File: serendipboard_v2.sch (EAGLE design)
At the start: 18 parts, among them IC1 TP4056, IC2 DW01A, Q1 FS8205A, Q2 DMP3056LSD, Q3 DMP3056LSD

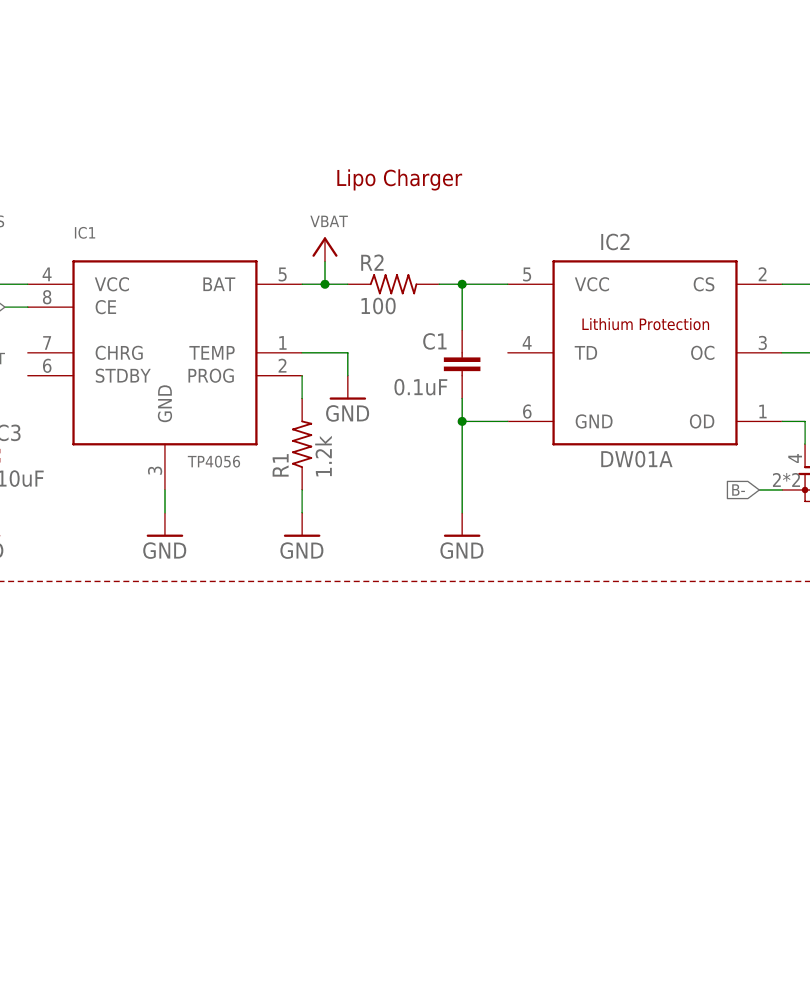
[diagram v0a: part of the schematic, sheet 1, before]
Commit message: Update serendipboard_v2.sch
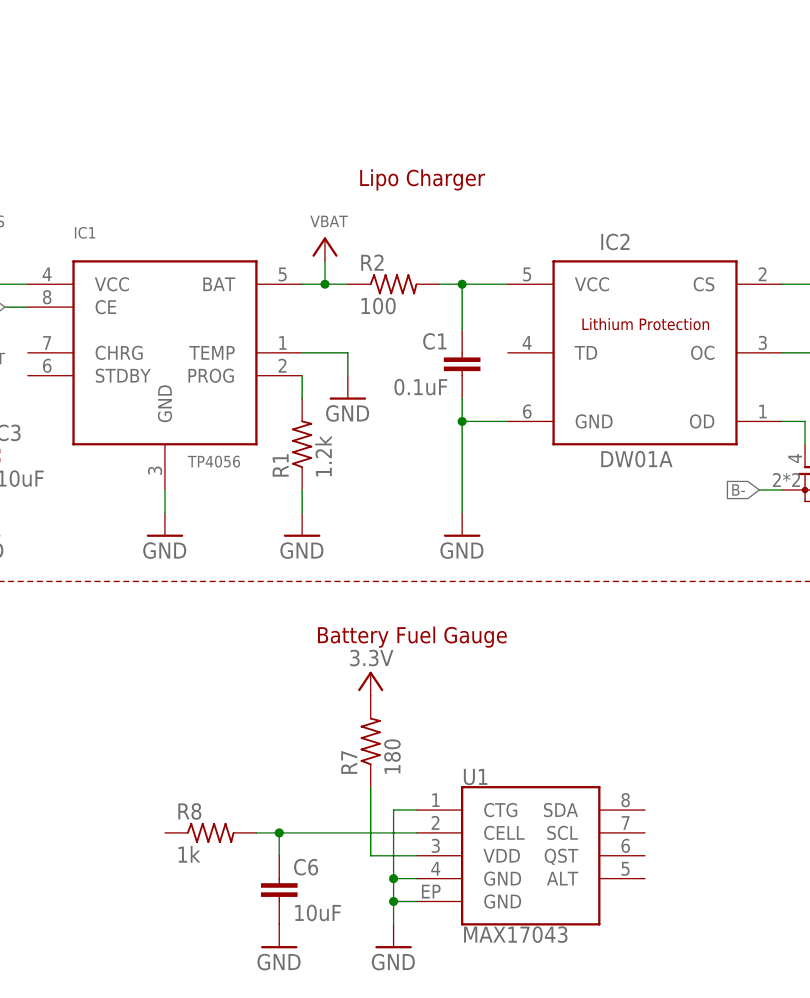
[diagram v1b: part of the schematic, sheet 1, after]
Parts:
- added C6: 10uF, rcl:C-EUC0805
- added R7: 180, rcl:R-US_R0805
- added R8: 1k, rcl:R-US_R0805
- added U1: MAX17043, SparkFun-IC-Power:MAX1704X
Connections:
- new net N$6: R7.1, U1.VDD
- new net N$7: C6.1, R8.2, U1.CELL
- net GND: now also C6.2, U1.CTG, U1.GND@4, U1.GND@EP
- net VCC: now also R7.2
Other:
- note added: "Battery Fuel Gauge"
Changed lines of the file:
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@@
 <layer number="112" name="tSilk" color="7" fill="1" visible="no" active="yes"/>
 <layer number="113" name="ReferenceLS" color="7" fill="1" visible="no" active="no"/>
+<layer number="114" name="Badge_Outline" color="7" fill="1" visible="yes" active="yes"/>
+<layer number="115" name="ReferenceISLANDS" color="7" fill="1" visible="yes" active="yes"/>
 <layer number="116" name="Patch_BOT" color="9" fill="4" visible="no" active="yes"/>
 <layer number="118" name="Rect_Pads" color="7" fill="1" visible="no" active="no"/>
@@
 <part name="P+10" library="supply1" library_urn="urn:adsk.eagle:library:371" deviceset="VCC" device="" value="V_oled"/>
 <part name="P+11" library="supply1" library_urn="urn:adsk.eagle:library:371" deviceset="VCC" device="" value="V_load"/>
+<part name="U1" library="SparkFun-IC-Power" library_urn="urn:adsk.eagle:library:526" deviceset="MAX1704X" device="" package3d_urn="urn:adsk.eagle:package:39055/1" value="MAX17043"/>
+<part name="C6" library="rcl" library_urn="urn:adsk.eagle:library:334" deviceset="C-EU" device="C0805" package3d_urn="urn:adsk.eagle:package:23617/2" value="10uF"/>
+<part name="R7" library="rcl" library_urn="urn:adsk.eagle:library:334" deviceset="R-US_" device="R0805" package3d_urn="urn:adsk.eagle:package:23553/2" value="180"/>
+<part name="GND10" library="supply1" library_urn="urn:adsk.eagle:library:371" deviceset="GND" device=""/>
+<part name="P+12" library="supply1" library_urn="urn:adsk.eagle:library:371" deviceset="VCC" device="" value="3.3V"/>
+<part name="R8" library="rcl" library_urn="urn:adsk.eagle:library:334" deviceset="R-US_" device="R0805" package3d_urn="urn:adsk.eagle:package:23553/2" value="1k"/>
+<part name="GND11" library="supply1" library_urn="urn:adsk.eagle:library:371" deviceset="GND" device=""/>
 </parts>
 <sheets>
 <sheet>
 <plain>
-<text x="68.58" y="177.8" size="1.778" layer="94" rot="R180">Lipo Charger</text>
+<text x="71.12" y="177.8" size="1.778" layer="94" rot="R180">Lipo Charger</text>
 <wire x1="0" y1="132.08" x2="134.62" y2="132.08" width="0.1524" layer="94" style="shortdash"/>
 <wire x1="134.62" y1="132.08" x2="134.62" y2="180.34" width="0.1524" layer="94" style="shortdash"/>
@@
 <wire x1="195.58" y1="132.08" x2="264.16" y2="132.08" width="0.1524" layer="94" style="shortdash"/>
 <text x="238.76" y="177.8" size="1.778" layer="94" rot="R180">3.3v Rail Control</text>
+<text x="73.66" y="127" size="1.778" layer="94" rot="R180">Battery Fuel Gauge</text>
 </plain>
 <instances>
@@
 <instance part="P+11" gate="VCC" x="248.92" y="149.86" smashed="yes" rot="R270">
 <attribute name="VALUE" x="251.46" y="147.32" size="1.27" layer="96" rot="R90"/>
+</instance>
+<instance part="U1" gate="G$1" x="76.2" y="101.6" smashed="yes">
+<attribute name="NAME" x="68.58" y="109.474" size="1.778" layer="95"/>
+<attribute name="VALUE" x="68.58" y="91.948" size="1.778" layer="96"/>
+</instance>
+<instance part="C6" gate="G$1" x="48.26" y="99.06" smashed="yes">
+<attribute name="NAME" x="49.784" y="99.441" size="1.778" layer="95"/>
+<attribute name="VALUE" x="49.784" y="94.361" size="1.778" layer="96"/>
+</instance>
+<instance part="R7" gate="G$1" x="58.42" y="114.3" smashed="yes" rot="R90">
+<attribute name="NAME" x="56.9214" y="110.49" size="1.778" layer="95" rot="R90"/>
+<attribute name="VALUE" x="61.722" y="110.49" size="1.778" layer="96" rot="R90"/>
+</instance>
+<instance part="GND10" gate="1" x="60.96" y="91.44" smashed="yes">
+<attribute name="VALUE" x="58.42" y="88.9" size="1.778" layer="96"/>
+</instance>
+<instance part="P+12" gate="VCC" x="58.42" y="121.92" smashed="yes">
+<attribute name="VALUE" x="60.96" y="124.46" size="1.778" layer="96" rot="R180"/>
+</instance>
+<instance part="R8" gate="G$1" x="40.64" y="104.14" smashed="yes">
+<attribute name="NAME" x="36.83" y="105.6386" size="1.778" layer="95"/>
+<attribute name="VALUE" x="36.83" y="100.838" size="1.778" layer="96"/>
+</instance>
+<instance part="GND11" gate="1" x="48.26" y="91.44" smashed="yes">
+<attribute name="VALUE" x="45.72" y="88.9" size="1.778" layer="96"/>
 </instance>
 </instances>
@@
 <wire x1="180.34" y1="139.7" x2="170.18" y2="139.7" width="0.1524" layer="91"/>
 <junction x="170.18" y="139.7"/>
+</segment>
+<segment>
+<pinref part="U1" gate="G$1" pin="CTG"/>
+<pinref part="GND10" gate="1" pin="GND"/>
+<wire x1="63.5" y1="106.68" x2="60.96" y2="106.68" width="0.1524" layer="91"/>
+<wire x1="60.96" y1="106.68" x2="60.96" y2="99.06" width="0.1524" layer="91"/>
+<pinref part="U1" gate="G$1" pin="GND@EP"/>
+<wire x1="60.96" y1="99.06" x2="60.96" y2="96.52" width="0.1524" layer="91"/>
+<wire x1="60.96" y1="96.52" x2="60.96" y2="93.98" width="0.1524" layer="91"/>
+<wire x1="63.5" y1="96.52" x2="60.96" y2="96.52" width="0.1524" layer="91"/>
+<junction x="60.96" y="96.52"/>
+<pinref part="U1" gate="G$1" pin="GND@4"/>
+<wire x1="63.5" y1="99.06" x2="60.96" y2="99.06" width="0.1524" layer="91"/>
+<junction x="60.96" y="99.06"/>
+</segment>
+<segment>
+<pinref part="C6" gate="G$1" pin="2"/>
+<pinref part="GND11" gate="1" pin="GND"/>
 </segment>
 </net>
@@
 <pinref part="P+11" gate="VCC" pin="VCC"/>
 </segment>
+<segment>
+<pinref part="R7" gate="G$1" pin="2"/>
+<pinref part="P+12" gate="VCC" pin="VCC"/>
+</segment>
 </net>
 <net name="CHARGER_EN" class="0">
@@
 </segment>
 </net>
+<net name="N$6" class="0">
+<segment>
+<pinref part="U1" gate="G$1" pin="VDD"/>
+<wire x1="63.5" y1="101.6" x2="58.42" y2="101.6" width="0.1524" layer="91"/>
+<wire x1="58.42" y1="101.6" x2="58.42" y2="109.22" width="0.1524" layer="91"/>
+<pinref part="R7" gate="G$1" pin="1"/>
+</segment>
+</net>
+<net name="N$7" class="0">
+<segment>
+<pinref part="R8" gate="G$1" pin="2"/>
+<pinref part="U1" gate="G$1" pin="CELL"/>
+<wire x1="45.72" y1="104.14" x2="48.26" y2="104.14" width="0.1524" layer="91"/>
+<pinref part="C6" gate="G$1" pin="1"/>
+<wire x1="48.26" y1="104.14" x2="63.5" y2="104.14" width="0.1524" layer="91"/>
+<wire x1="48.26" y1="101.6" x2="48.26" y2="104.14" width="0.1524" layer="91"/>
+<junction x="48.26" y="104.14"/>
+</segment>
+</net>

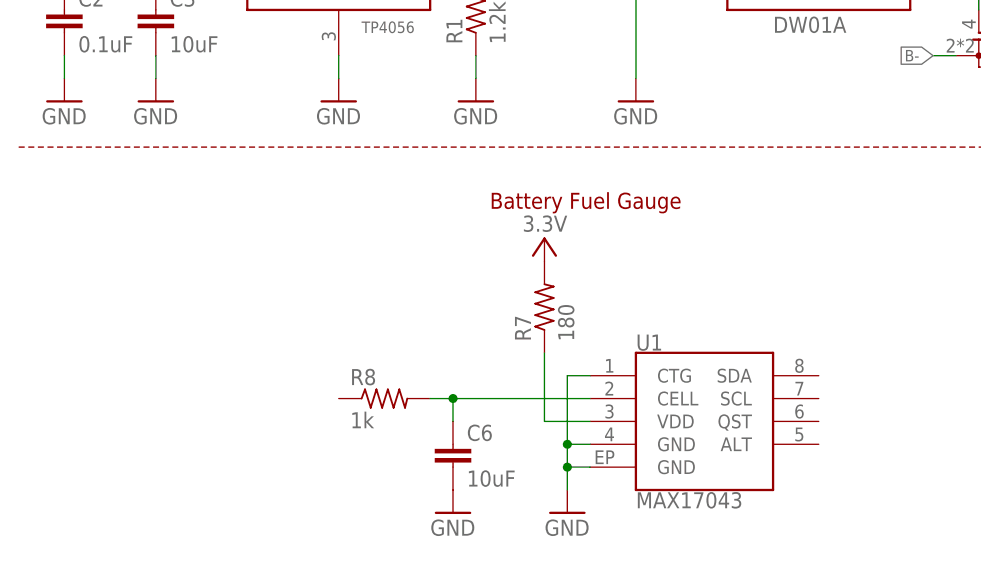
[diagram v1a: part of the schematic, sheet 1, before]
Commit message: Update serendipboard_v2.sch
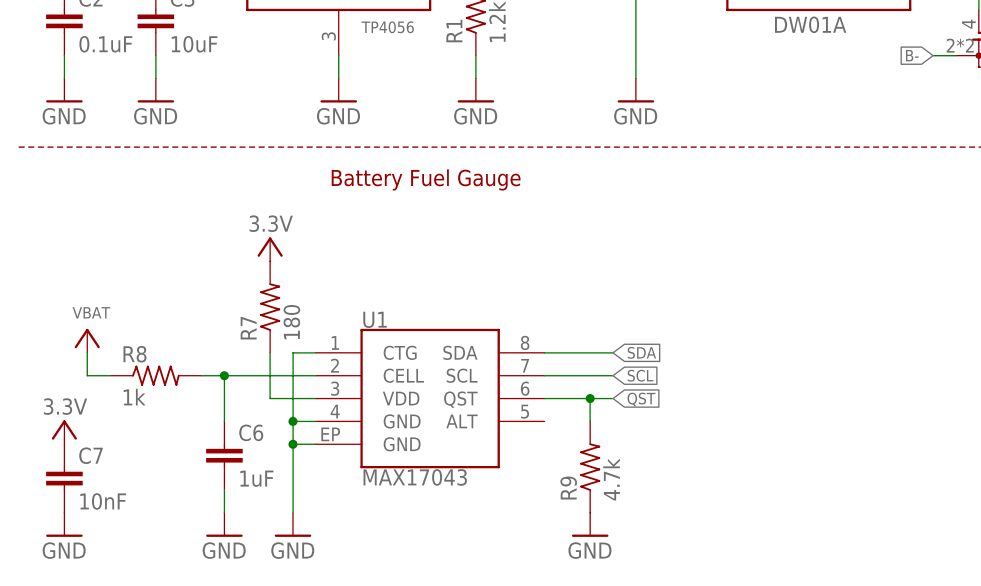
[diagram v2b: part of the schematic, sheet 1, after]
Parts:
- added C7: 10nF, rcl:C-EUC0805
- added R9: 4.7k, rcl:R-US_R0805
- C6: value 10uF -> 1uF
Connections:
- new net QST: R9.2, U1.QST
- new net SCL: U1.SCL
- new net SDA: U1.SDA
- net GND: now also C7.2, R9.1
- net VCC: now also C7.1, R8.1
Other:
- moved on the sheet: C6, R7, R8, U1

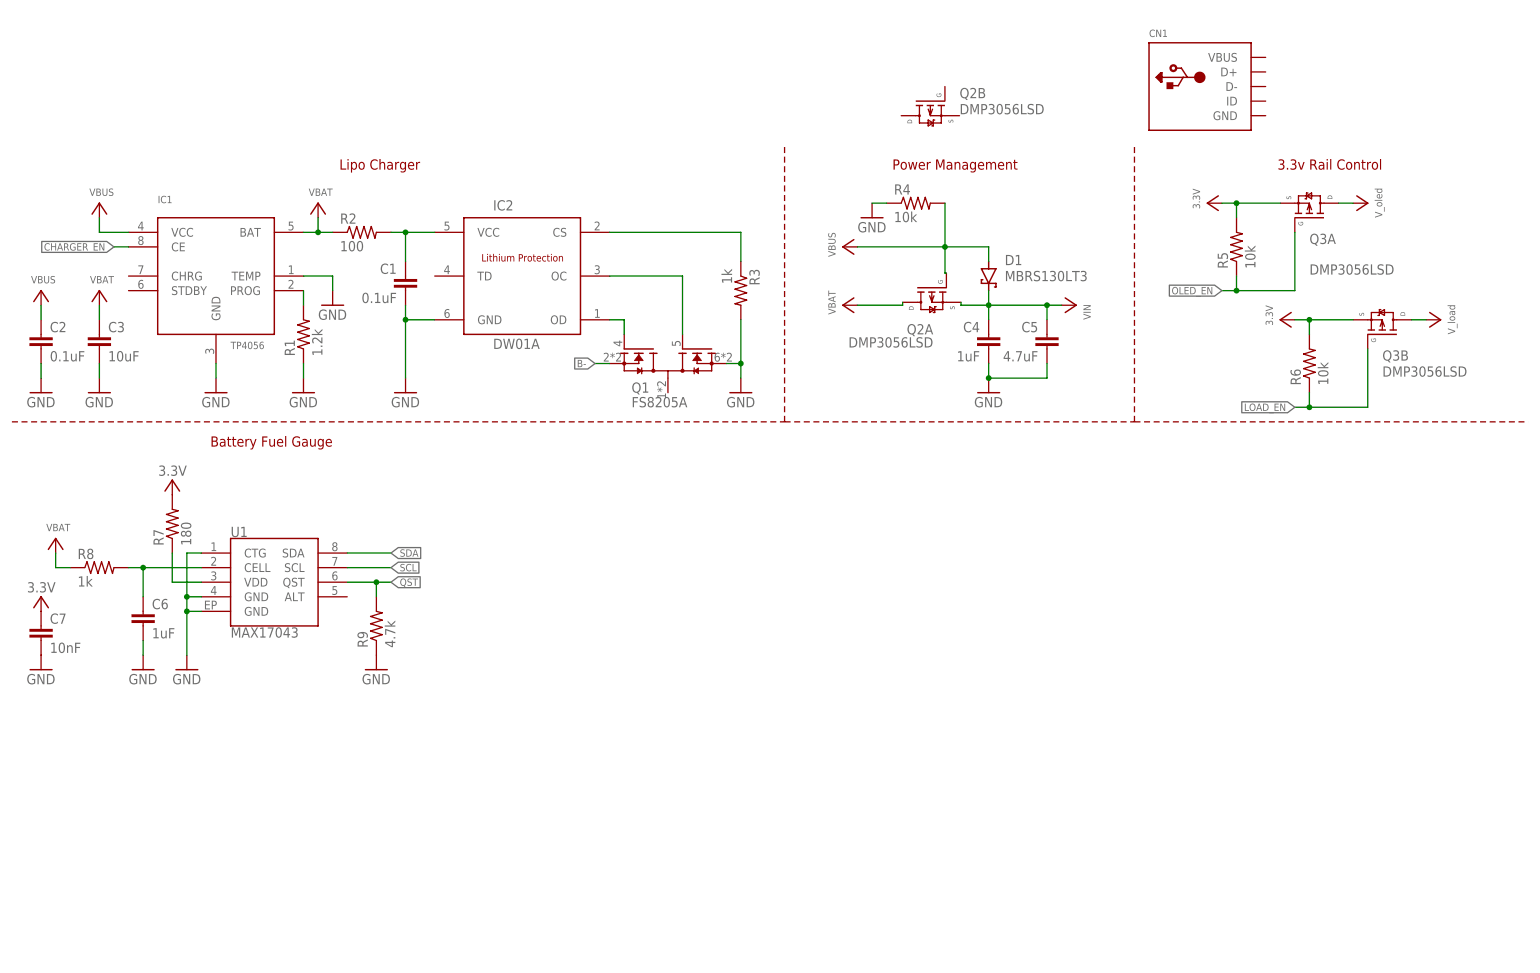
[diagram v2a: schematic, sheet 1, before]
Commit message: Update serendipboard_v2.sch
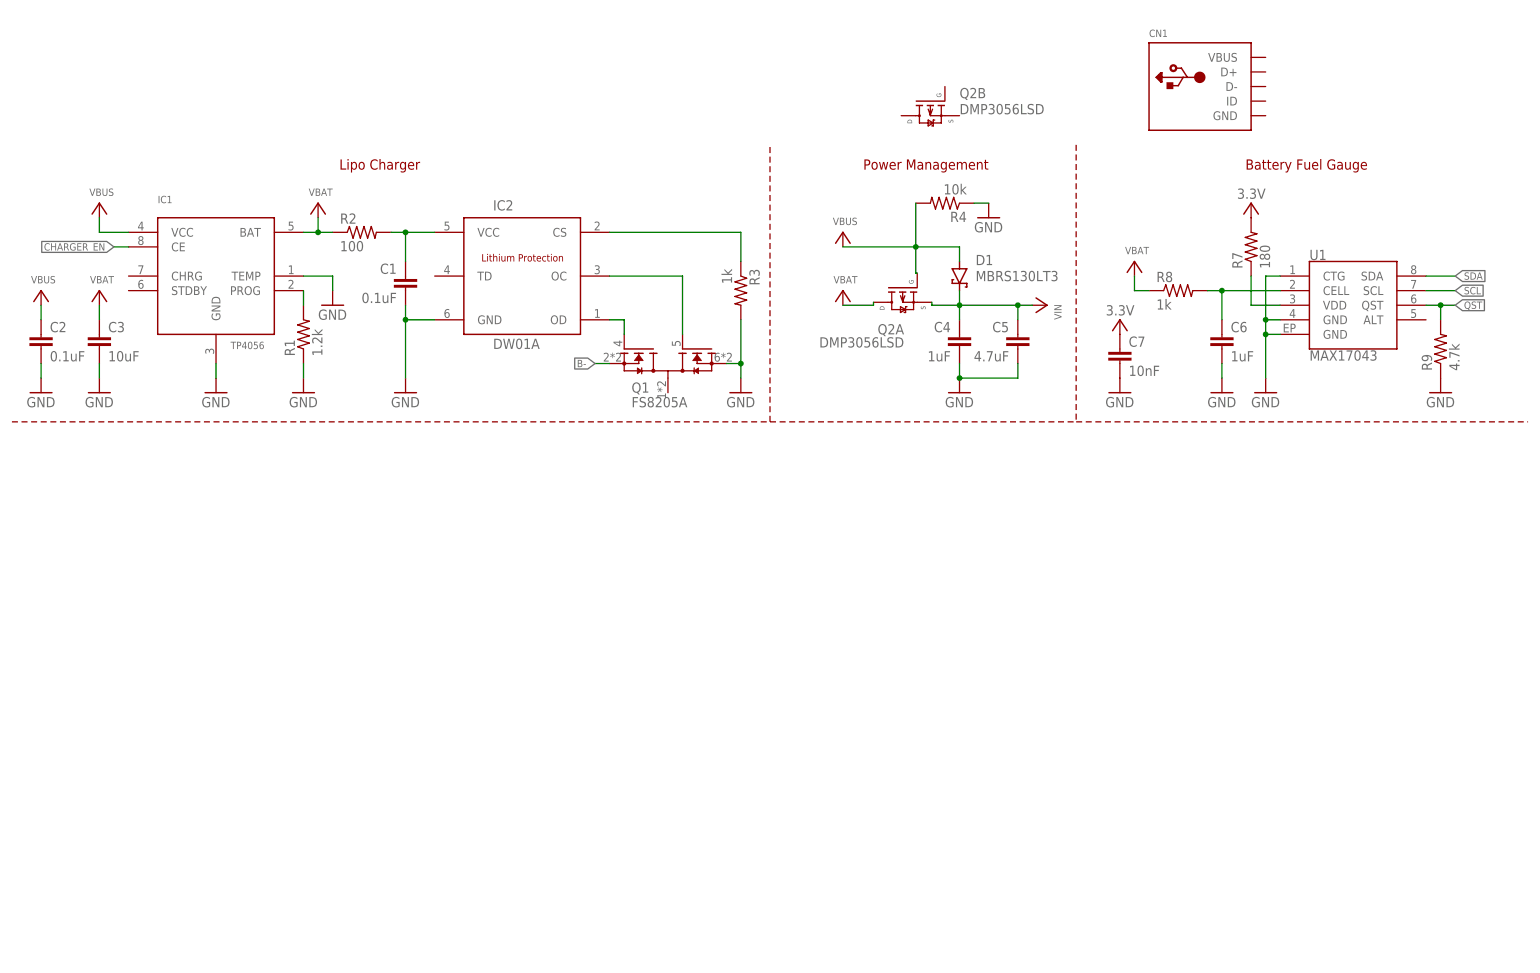
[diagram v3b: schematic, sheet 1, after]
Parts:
- removed Q3: DMP3056LSD, transistor FET special:DMP3056LSD
- removed R5, R6: 10k, rcl:R-US_R0805
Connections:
- removed net LOAD_EN: Q3B.G, R6.1
- removed net OLED_EN: Q3A.G, R5.1
- net VCC: no longer Q3A.D, Q3A.S, Q3B.D, Q3B.S, R5.2, R6.2
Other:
- note removed: "3.3v Rail Control"
- moved on the sheet: C4, C5, C6, C7, D1, Q2A, R4, R7, R8, R9, U1

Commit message: Update serendipboard_v2.sch
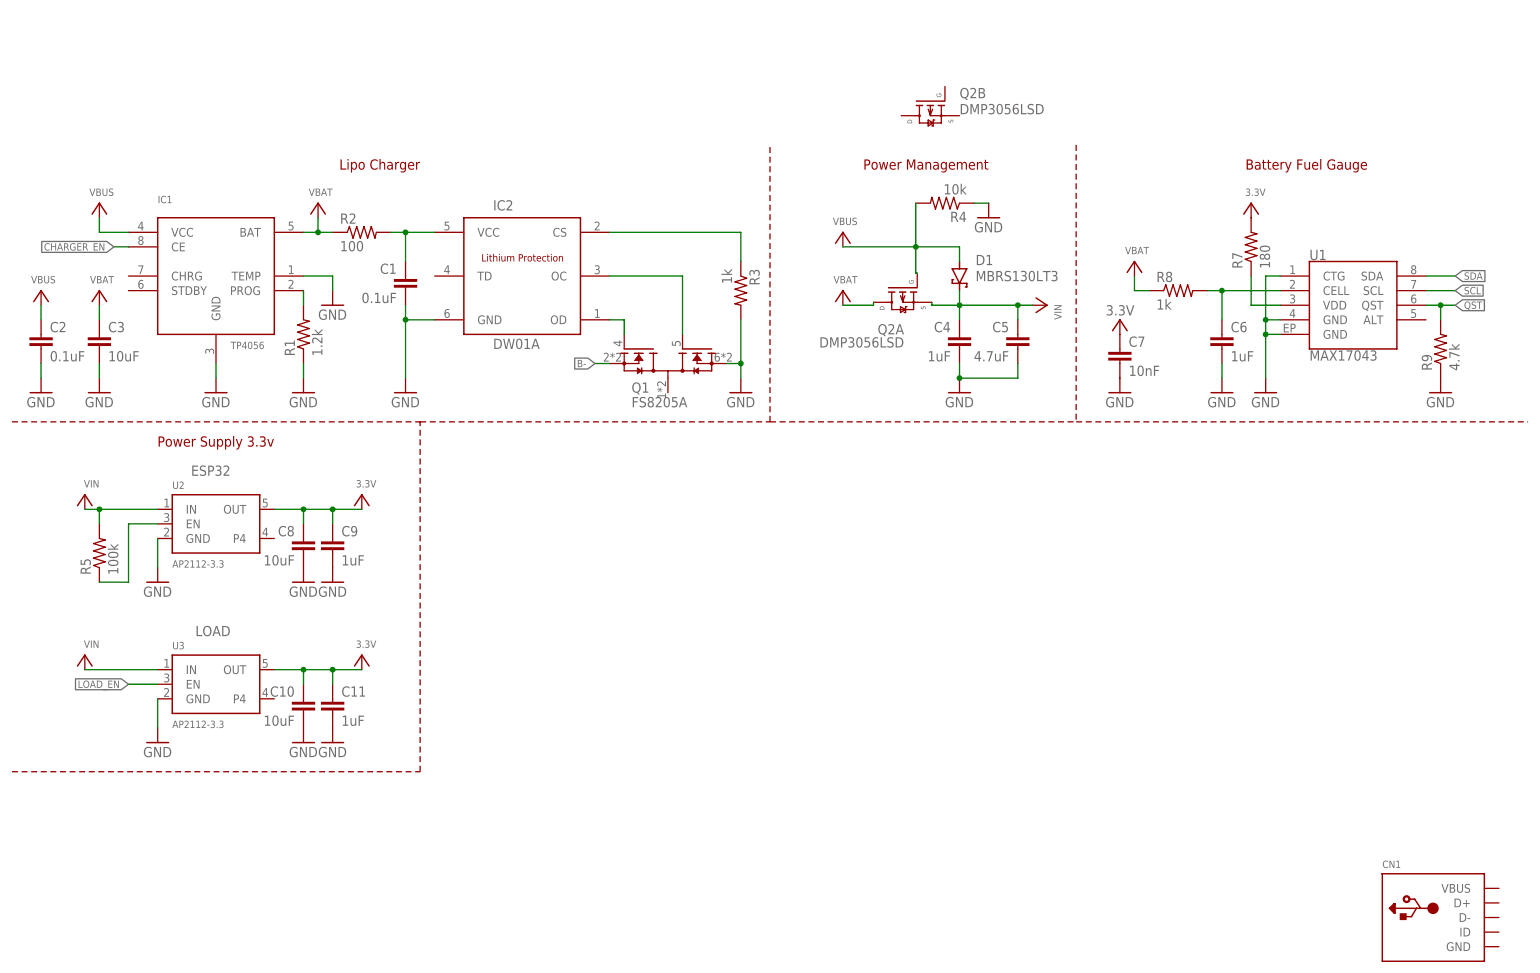
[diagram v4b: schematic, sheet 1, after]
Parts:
- added C10, C8: 10uF, rcl:C-EUC0805
- added C11, C9: 1uF, rcl:C-EUC0805
- added R5: 100k, rcl:R-US_R0805
- added U2, U3: AP2112-3.3, microbuilder:VREG_SOT23-5
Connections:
- new net LOAD_EN: U3.EN
- new net N$8: R5.1, U2.EN
- net GND: now also C10.2, C11.2, C8.2, C9.2, U2.GND, U3.GND
- net VCC: now also C10.1, C11.1, C8.1, C9.1, R5.2, U2.IN, U2.OUT, U3.IN, U3.OUT
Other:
- note added: "ESP32"
- note added: "LOAD"
- note added: "Power Supply 3.3v"
- moved on the sheet: CN1
